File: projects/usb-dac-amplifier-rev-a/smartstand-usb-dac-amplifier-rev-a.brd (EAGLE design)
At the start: 174.7 x 136 mm, 247 parts, among them J1 PJ-002A, J2 292304-1, J3 NRJ6HH, J4 PJRAN2X1U01AUX, J5 T1M-5POS, U1 XUF208-256-TQ64, U10 TPS3702, U11 PCM5102A, U12 SZNUD3124, U13 NJM2068M, U14 NJM4556AM, U15 NJM4556AM, U16 TS5A3159DBV, U17 SN74LVC3G34DCU, U18 TPD2E007DCK, U19 TPD2E007DCK, U2 TPD4E02B04DQA, U3 TPS563200DDC, U4 TPS7A8300RGW, U5 TPS563200DDC, U6 TPS7A8300RGW, U7 TPS7A8300RGW, U8 TPS7A4701RGW, U9 TPS7A3301RGW, X1 24MHz, X2 22.5792MHz, X3 24.576MHz

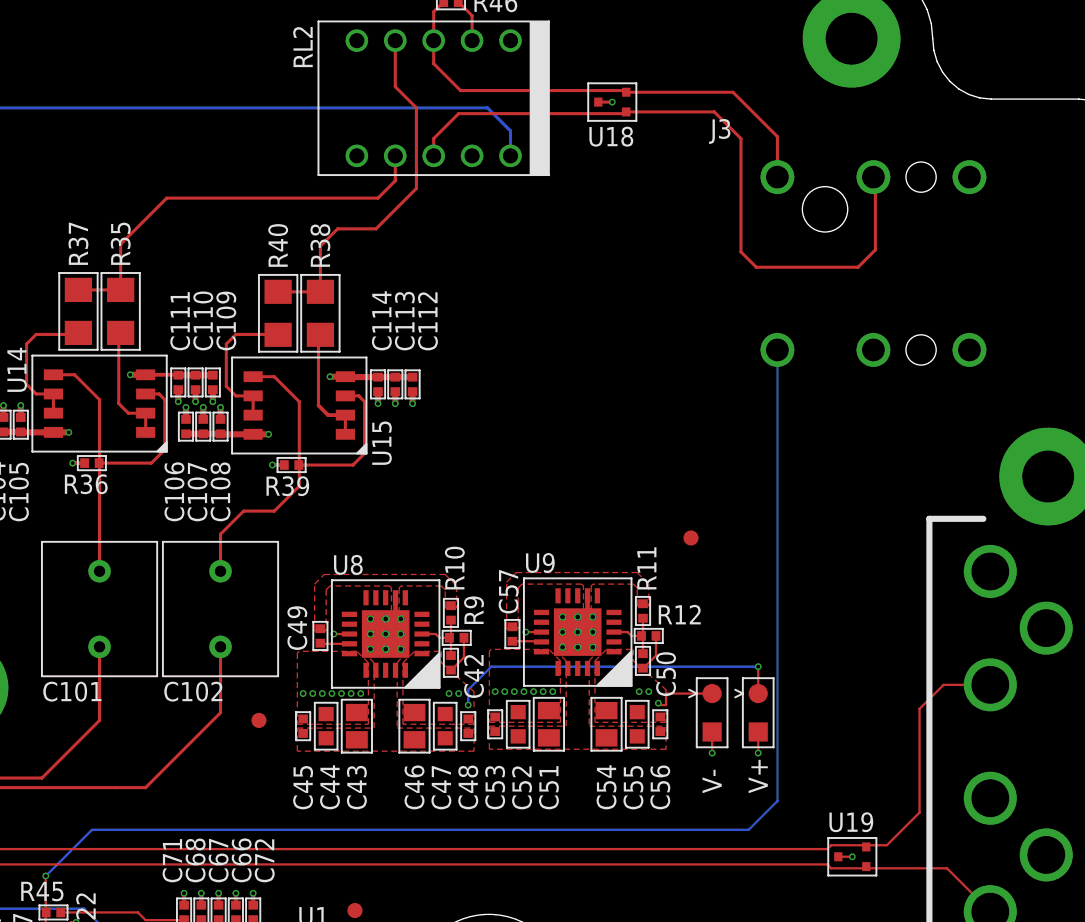
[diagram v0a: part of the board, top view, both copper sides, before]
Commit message: Shift headphone jack outwards to before more flush.
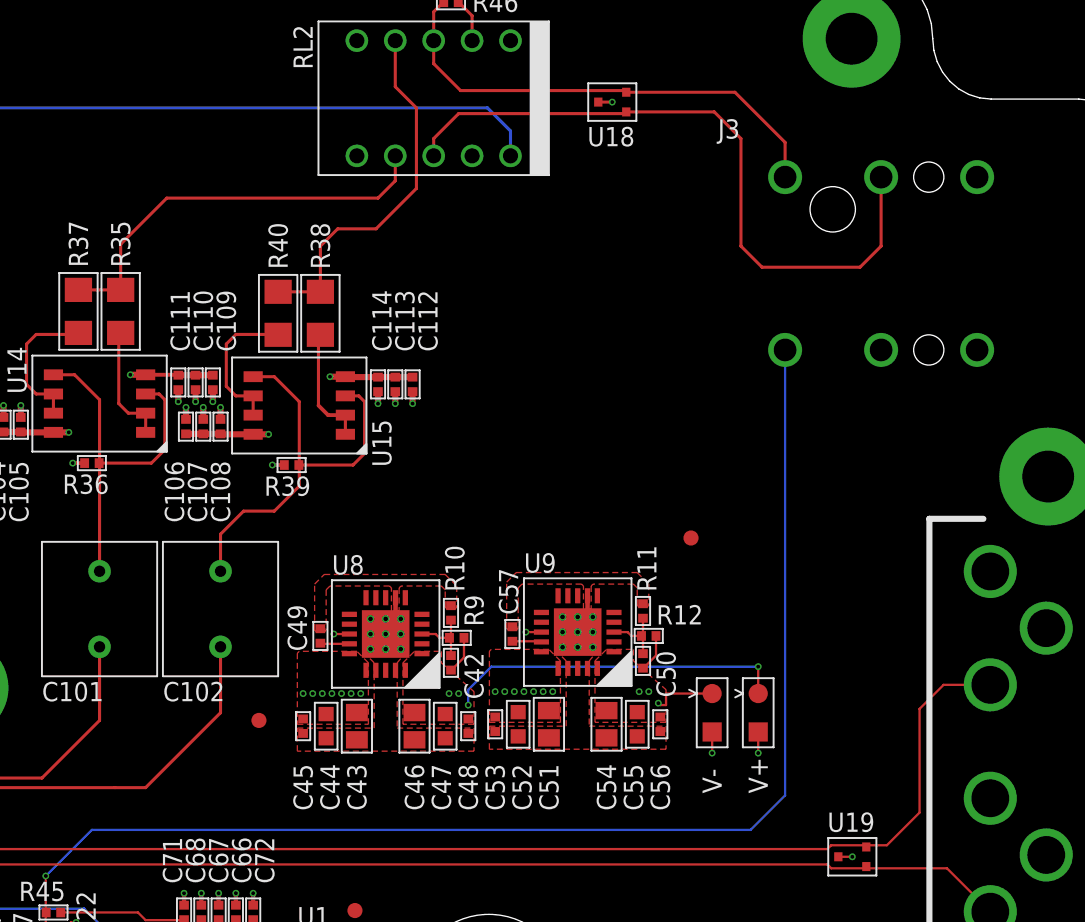
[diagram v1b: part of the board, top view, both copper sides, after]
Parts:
- moved J3 0.51 mm to (77.7, 46.6)
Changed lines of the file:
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@@
 <attribute name="NAME" x="78.613" y="-42.926" size="1.27" layer="25" font="vector" ratio="12"/>
 </element>
-<element name="J3" library="neutrik" package="NRJ6HH" value="NRJ6HH" x="77.216" y="46.609" smashed="yes">
-<attribute name="NAME" x="66.421" y="56.388" size="1.27" layer="25" font="vector" ratio="12"/>
-<attribute name="PN" value="NRJ6HH" x="77.216" y="46.609" size="1.778" layer="27" display="off"/>
+<element name="J3" library="neutrik" package="NRJ6HH" value="NRJ6HH" x="77.724" y="46.609" smashed="yes">
+<attribute name="NAME" x="66.929" y="56.388" size="1.27" layer="25" font="vector" ratio="12"/>
+<attribute name="PN" value="NRJ6HH" x="77.724" y="46.609" size="1.778" layer="27" display="off"/>
 </element>
 <element name="JP2" library="pinhead" package="2X10" value="" x="-15.621" y="22.352" smashed="yes">
@@
 <contactref element="R46" pad="2"/>
 <wire x1="48.133" y1="62.865" x2="48.133" y2="61.341" width="0.2032" layer="1"/>
-<wire x1="70.866" y1="56.515" x2="70.866" y2="53.839" width="0.2032" layer="1"/>
 <wire x1="48.796" y1="65.405" x2="48.768" y2="65.405" width="0.1524" layer="1"/>
 <wire x1="48.768" y1="65.405" x2="48.133" y2="64.77" width="0.2032" layer="1"/>
@@
 <wire x1="49.911" y1="59.563" x2="60.757" y2="59.563" width="0.2032" layer="1"/>
 <wire x1="60.757" y1="59.563" x2="60.869" y2="59.451" width="0.2032" layer="1"/>
-<wire x1="60.869" y1="59.451" x2="67.93" y2="59.451" width="0.2032" layer="1"/>
-<wire x1="67.93" y1="59.451" x2="70.866" y2="56.515" width="0.2032" layer="1"/>
+<wire x1="60.869" y1="59.451" x2="68.057" y2="59.451" width="0.2032" layer="1"/>
+<wire x1="68.057" y1="59.451" x2="71.374" y2="56.134" width="0.2032" layer="1"/>
+<wire x1="71.374" y1="56.134" x2="71.374" y2="53.839" width="0.2032" layer="1"/>
 </signal>
 <signal name="N$29">
@@
 <contactref element="RL2" pad="P$8"/>
 <wire x1="48.133" y1="55.245" x2="48.133" y2="56.388" width="0.2032" layer="1"/>
-<wire x1="68.453" y1="48.895" x2="69.469" y2="47.879" width="0.2032" layer="1"/>
-<wire x1="69.469" y1="47.879" x2="76.2" y2="47.879" width="0.2032" layer="1"/>
-<wire x1="76.2" y1="47.879" x2="77.343" y2="49.022" width="0.2032" layer="1"/>
-<wire x1="77.343" y1="49.022" x2="77.343" y2="53.712" width="0.2032" layer="1"/>
-<wire x1="77.343" y1="53.712" x2="77.216" y2="53.839" width="0.2032" layer="1"/>
+<wire x1="68.453" y1="49.276" x2="69.85" y2="47.879" width="0.2032" layer="1"/>
+<wire x1="69.85" y1="47.879" x2="76.327" y2="47.879" width="0.2032" layer="1"/>
 <contactref element="U18" pad="1"/>
 <wire x1="48.133" y1="56.388" x2="49.784" y2="58.039" width="0.2032" layer="1"/>
@@
 <wire x1="60.869" y1="58.151" x2="66.69" y2="58.151" width="0.2032" layer="1"/>
 <wire x1="66.69" y1="58.151" x2="68.453" y2="56.388" width="0.2032" layer="1"/>
-<wire x1="68.453" y1="56.388" x2="68.453" y2="48.895" width="0.2032" layer="1"/>
+<wire x1="68.453" y1="56.388" x2="68.453" y2="49.276" width="0.2032" layer="1"/>
+<wire x1="77.724" y1="53.839" x2="77.724" y2="49.276" width="0.2032" layer="1"/>
+<wire x1="77.724" y1="49.276" x2="76.327" y2="47.879" width="0.2032" layer="1"/>
 </signal>
 <signal name="N$64">
@@
 <contactref element="R45" pad="1"/>
 <contactref element="R47" pad="1"/>
-<wire x1="70.866" y1="42.409" x2="70.866" y2="12.573" width="0.1524" layer="16"/>
-<wire x1="70.866" y1="12.573" x2="68.961" y2="10.668" width="0.1524" layer="16"/>
-<wire x1="68.961" y1="10.668" x2="25.527" y2="10.668" width="0.1524" layer="16"/>
+<wire x1="71.374" y1="12.954" x2="69.088" y2="10.668" width="0.1524" layer="16"/>
+<wire x1="69.088" y1="10.668" x2="25.527" y2="10.668" width="0.1524" layer="16"/>
 <wire x1="25.527" y1="10.668" x2="22.479" y2="7.62" width="0.1524" layer="16"/>
 <via x="22.479" y="7.62" extent="1-16" drill="0.254"/>
@@
 <wire x1="22.479" y1="4.036" x2="22.479" y2="5.179" width="0.1524" layer="1"/>
 <wire x1="22.479" y1="5.179" x2="22.507" y2="5.207" width="0.1524" layer="1"/>
+<wire x1="71.374" y1="42.409" x2="71.374" y2="12.954" width="0.1524" layer="16"/>
 </signal>
 <signal name="N$62">
